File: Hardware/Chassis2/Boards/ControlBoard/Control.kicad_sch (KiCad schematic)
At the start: 41 parts, among them IC4 CY15B102Q-SXET, U1 STM32H723ZGTx, Y1 8MHz

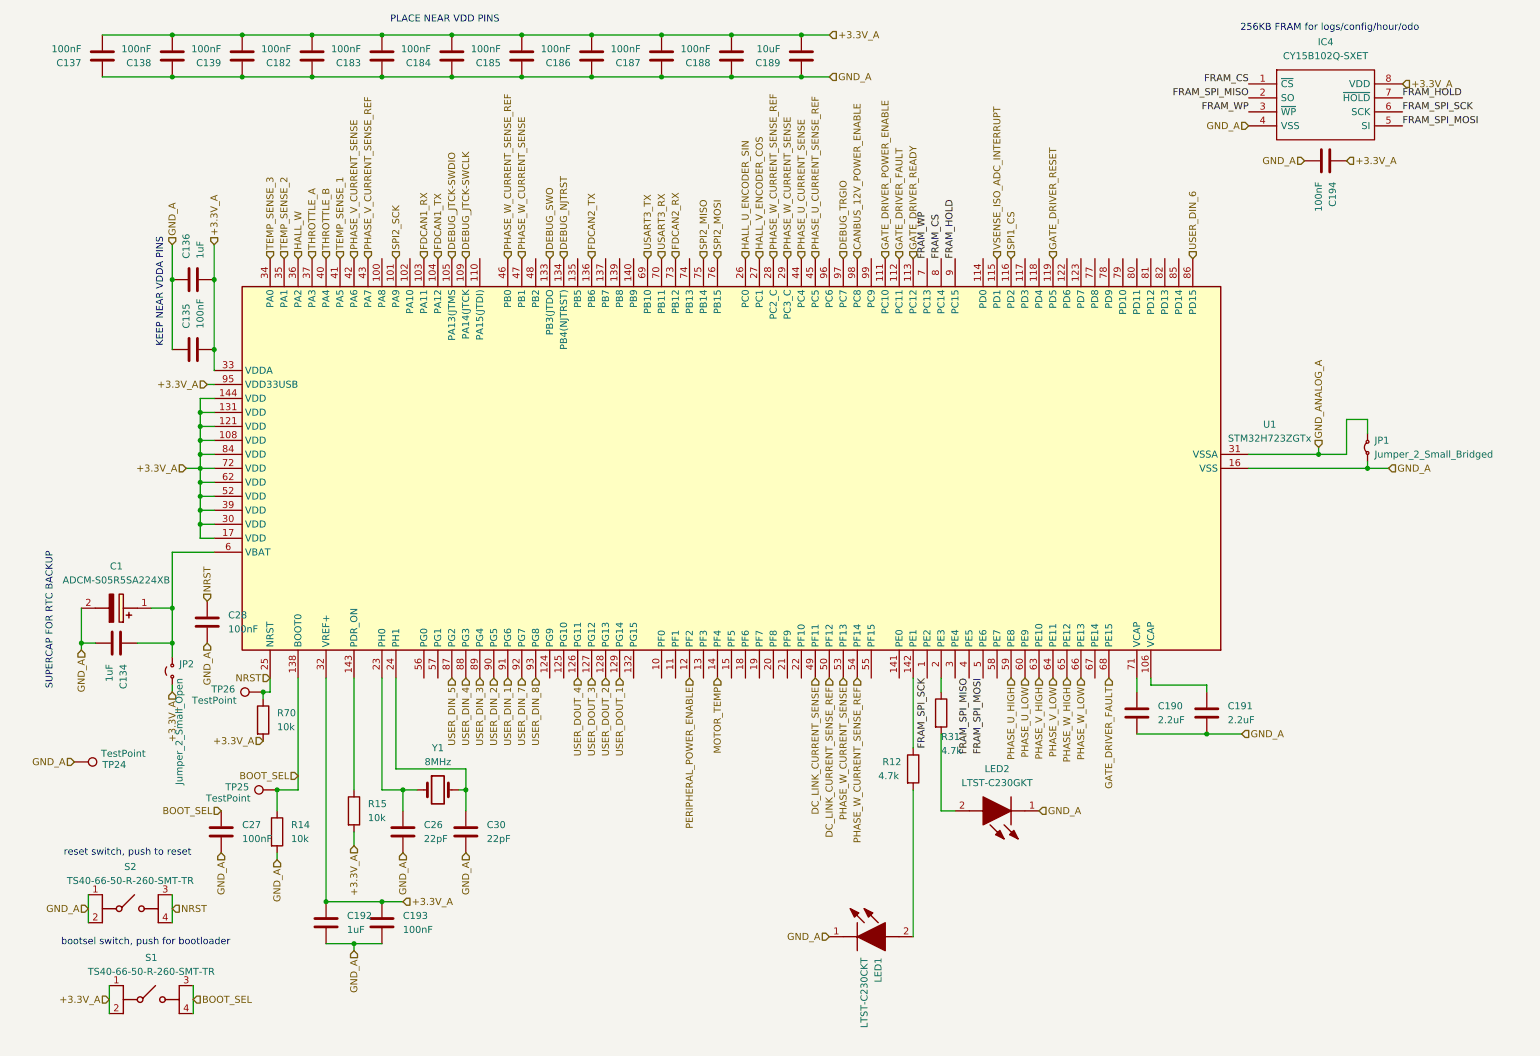
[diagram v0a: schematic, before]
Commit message: update hw revision 7
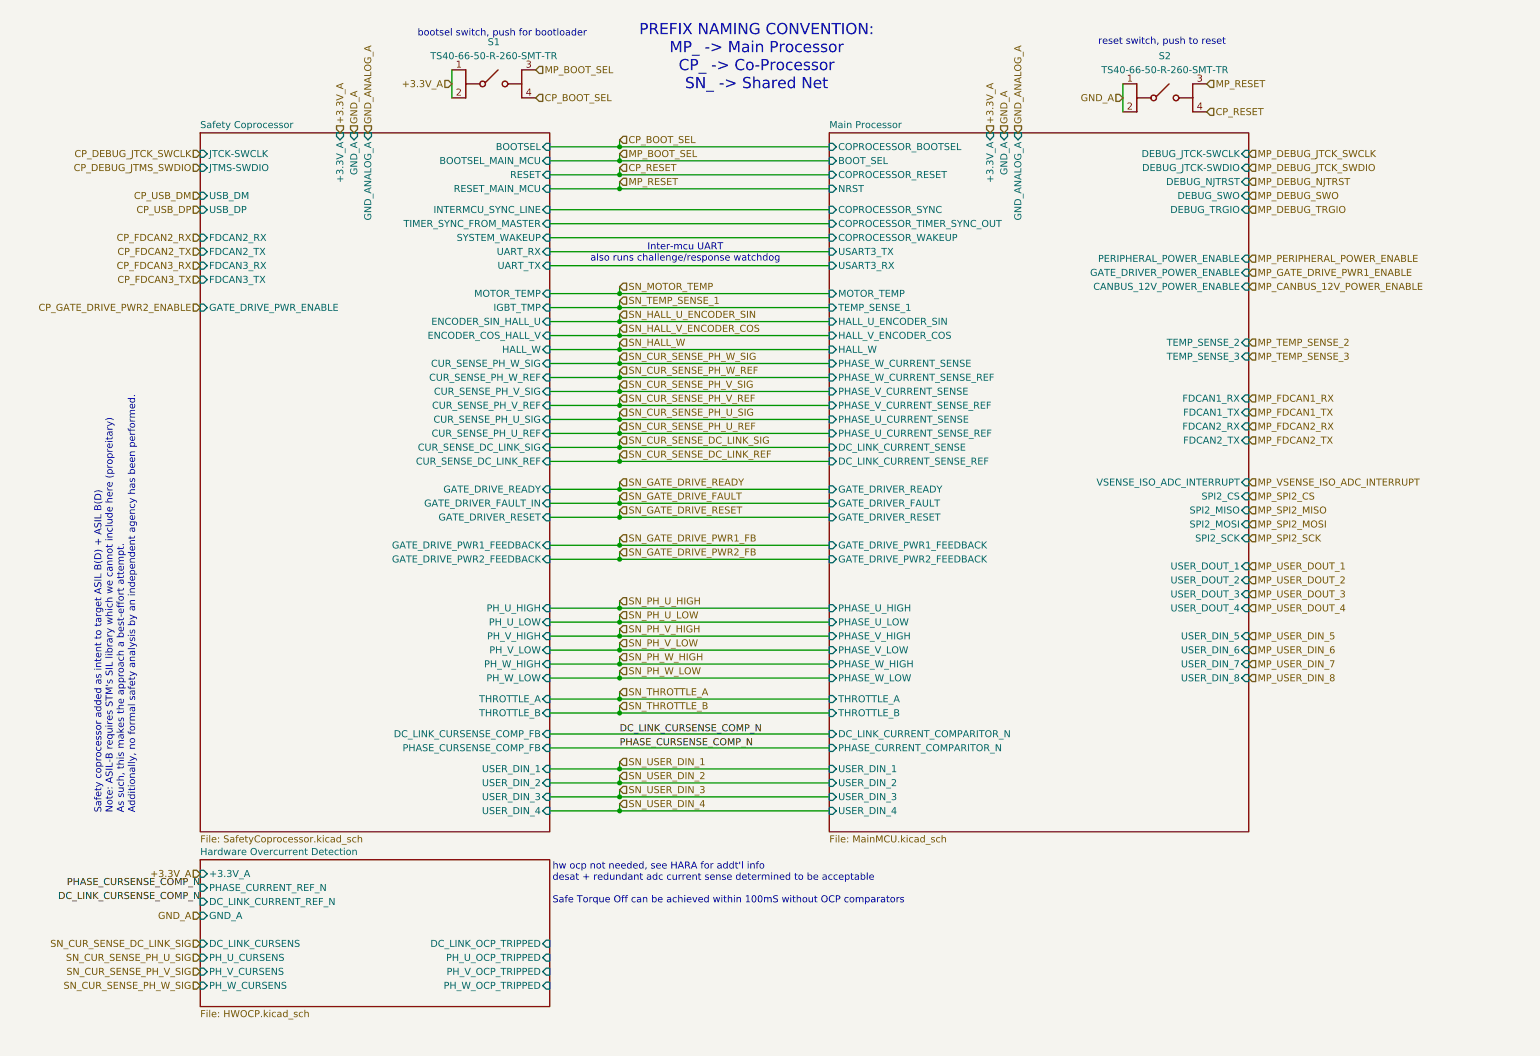
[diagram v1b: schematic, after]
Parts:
- removed C1: ADCM-S05R5SA224XB, ADCMS05R5SA224XB, symbol InverterCom:ADCM-S05R5SA224XB
- removed C134, C136, C192: 1uF, Capacitor_SMD:C_1210_3225Metric_Pad1.33x2.70mm_HandSolder, symbol Device:C
- removed C135, C137, C138, C139, C182, C183, C184, C185, C186, C187, C188, C193, C194, C27, C28: 100nF, Capacitor_SMD:C_1210_3225Metric_Pad1.33x2.70mm_HandSolder, symbol Device:C
- removed C189: 10uF, Capacitor_SMD:C_1210_3225Metric_Pad1.33x2.70mm_HandSolder, symbol Device:C
- removed C190, C191: 2.2uF, Capacitor_SMD:C_1210_3225Metric_Pad1.33x2.70mm_HandSolder, symbol Device:C
- removed C26, C30: 22pF, Capacitor_SMD:C_1210_3225Metric_Pad1.33x2.70mm_HandSolder, symbol Device:C
- removed IC4: CY15B102Q-SXET, SOIC127P800X203-8N, symbol InverterCom:CY15B102Q-SXET
- removed JP1: Jumper_2_Small_Bridged, Jumper:SolderJumper-2_P1.3mm_Bridged_Pad1.0x1.5mm, symbol Jumper:Jumper_2_Small_Bridged
- removed JP2: Jumper_2_Small_Open, Jumper:SolderJumper-2_P1.3mm_Open_RoundedPad1.0x1.5mm, symbol Jumper:Jumper_2_Small_Open
- removed LED1: LTST-C230CKT, LEDC3216X120N, symbol InverterCom:LTST-C230CKT
- removed LED2: LTST-C230GKT, LEDC3216X120N, symbol InverterCom:LTST-C230GKT
- removed R12, R31: 4.7k, Resistor_SMD:R_1210_3225Metric_Pad1.30x2.65mm_HandSolder, symbol Device:R
- removed R14, R15, R70: 10k, Resistor_SMD:R_1210_3225Metric_Pad1.30x2.65mm_HandSolder, symbol Device:R
- removed TP24, TP25, TP26: TestPoint, TestPoint:TestPoint_Loop_D2.54mm_Drill1.5mm_Beaded, symbol Connector:TestPoint
- removed U1: STM32H723ZGTx, Package_QFP:LQFP-144_20x20mm_P0.5mm, symbol MCU_ST_STM32H7:STM32H723ZGTx
- removed Y1: 8MHz, Crystal:Crystal_HC49-4H_Vertical, symbol Device:Crystal
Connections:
- net BOOT_SEL renamed CP_BOOT_SEL
- net CP_BOOT_SEL: no longer S1.3 (NO_1)
- net NRST renamed CP_RESET
- net CP_RESET: no longer S2.3 (NO_1)
- new net MP_BOOT_SEL: S1.3 (NO_1)
- new net MP_RESET: S2.3 (NO_1)
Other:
- added sheet Hardware Overcurrent Detection (HWOCP.kicad_sch)
- added sheet Main Processor (MainMCU.kicad_sch)
- added sheet Safety Coprocessor (SafetyCoprocessor.kicad_sch)
- note added: "Inter-mcu UART also runs challenge/response watchdog"
- note added: "PREFIX NAMING CONVENTION: MP_ -> Main Processor CP_ -> Co-Processor SN_ -> Shared Net"
- note added: "Safety coprocessor added as intent to target ASIL B(D) + ASIL B(D) Note: ASIL-B requires STM's SIL library which we cannot include here (propreitary) As such, this makes the approach a best-effort attempt. Additionally, no formal safety analysis by an independent agency has been performed."
- note added: "hw ocp not needed, see HARA for addt'l info desat + redundant adc current sense determined to be acceptable Safe Torque Off can be achieved within 100mS without OCP comparators"
- note removed: "256KB FRAM for logs/config/hour/odo"
- note removed: "KEEP NEAR VDDA PINS"
- note removed: "PLACE NEAR VDD PINS"
- note removed: "SUPERCAP FOR RTC BACKUP"
- company: (none) -> Corzine Lab, University of California, Santa Cruz
- title: (none) -> Open Inverter Platform - Control Board
- moved on the sheet: S1, S2

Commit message: eod 2026-07-08
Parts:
- S1, S2: footprint TS406650R260SMTTR -> InverterCom:TS406650R260SMTTR
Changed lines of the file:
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@@
 			)
 		)
-		(property "Footprint" "TS406650R260SMTTR"
+		(property "Footprint" "InverterCom:TS406650R260SMTTR"
 			(at 101.6 120.32 0)
 			(hide yes)
@@
 			)
 		)
-		(property "Footprint" "TS406650R260SMTTR"
+		(property "Footprint" "InverterCom:TS406650R260SMTTR"
 			(at 223.52 122.86 0)
 			(hide yes)
